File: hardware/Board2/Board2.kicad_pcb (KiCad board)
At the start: 4 copper layers, 54.1 x 63.2 mm, 5 parts, among them J1 Conn_01x02, J2 Conn_01x08, J3 OUT, J4 Conn_01x02

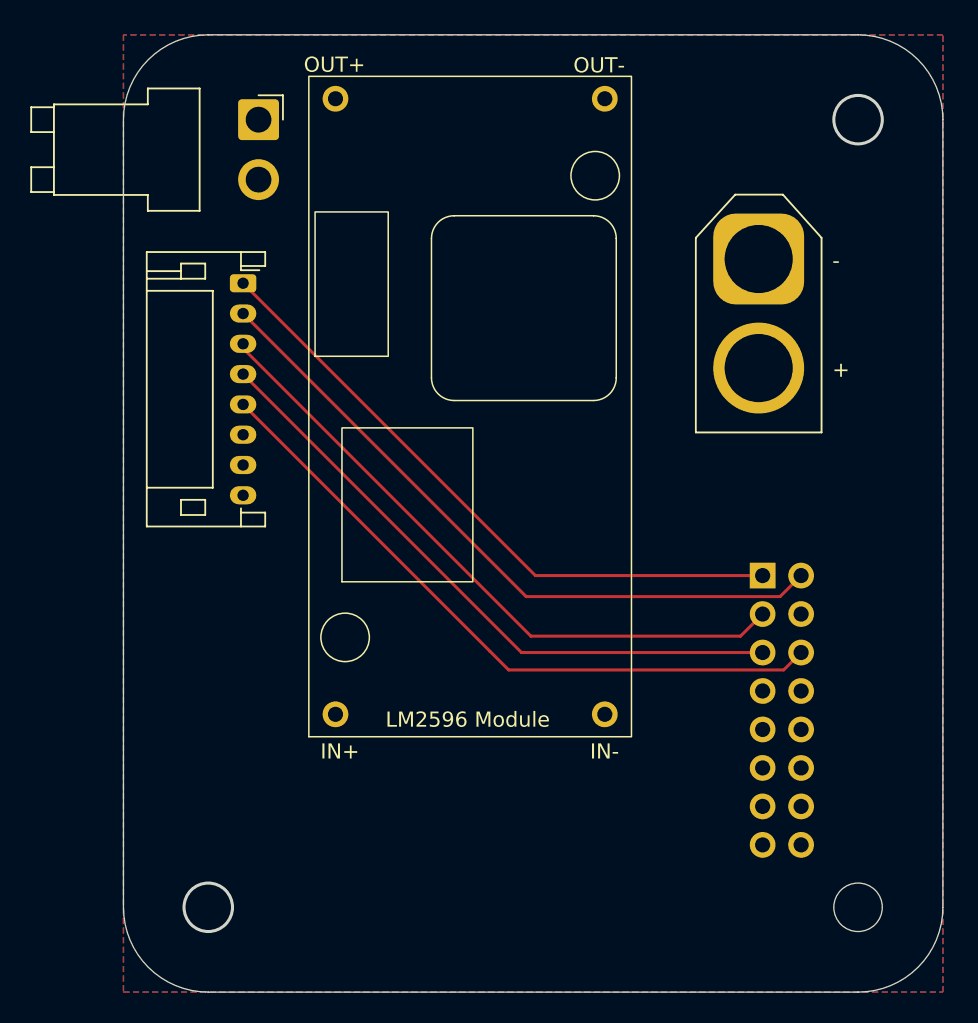
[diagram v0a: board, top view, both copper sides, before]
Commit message: Maybe done boards?
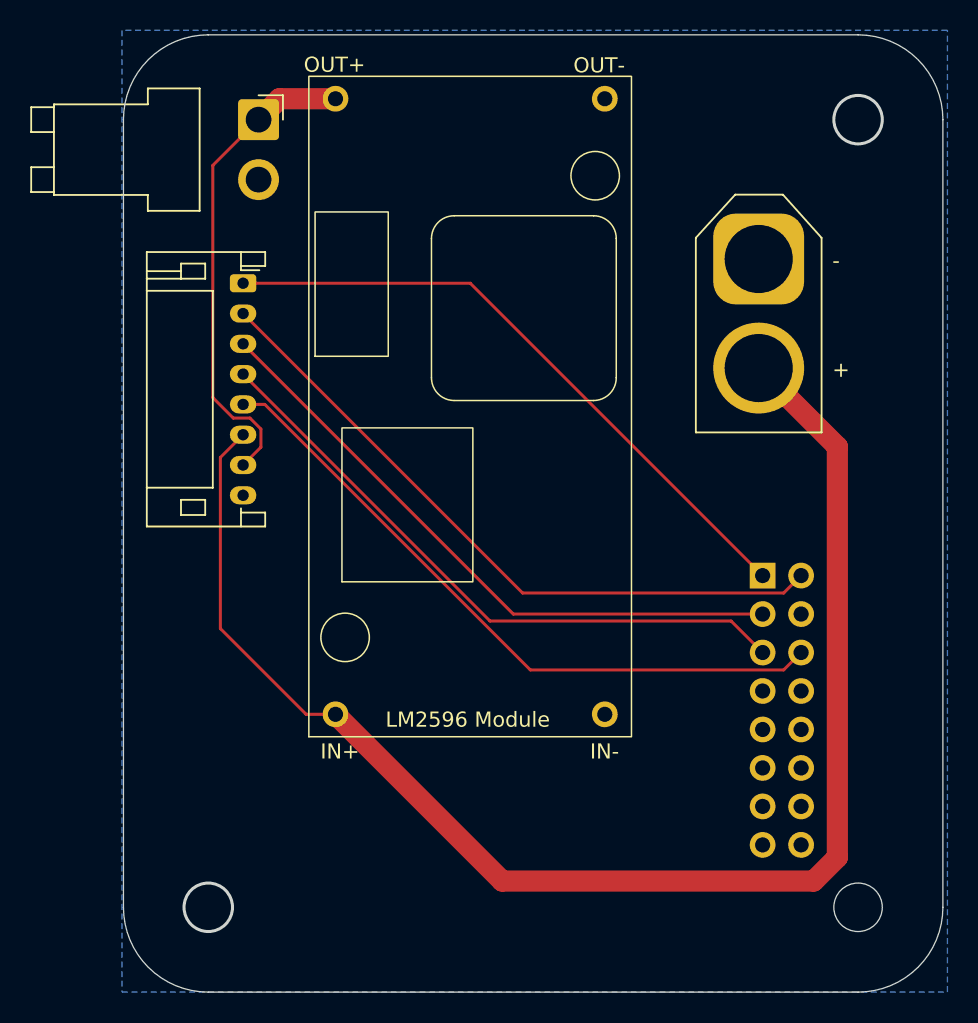
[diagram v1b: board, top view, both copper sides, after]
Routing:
- net +BATT: track 0.00 -> 96.2 mm
- net Earth: track 81.6 -> 0.00 mm
- net VCC: track 0.00 -> 32.1 mm
- net /B2: track 43.1 -> 41.7 mm
- added copper zone on B.Cu, net Earth
- removed copper zone on F.Cu, net +BATT
- removed copper zone on In1.Cu, net Earth
- removed copper zone on In2.Cu, net Earth
- removed copper zone on B.Cu, net VCC
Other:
- copper layers 4 -> 2
